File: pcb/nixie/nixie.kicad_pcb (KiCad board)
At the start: 2 copper layers, 144 x 117 mm, 49 parts, among them J1 Conn_01x32, J2 Conn_01x02, J3 Conn_01x32, J4 Conn_01x32, J5 Conn_01x32, P1 TTL_232R_3V3, Q1 Q_NMOS_DGS, U1 LM317EMP, U10 nixie_8422, U11 nixie_8422, U12 nixie_8422, U2 ESP-WROOM-32, U3 TACTILE, U4 TACTILE, U5 nixie_8422, U6 HV5530, U7 HV5530, U8 nixie_8422, U9 nixie_8422

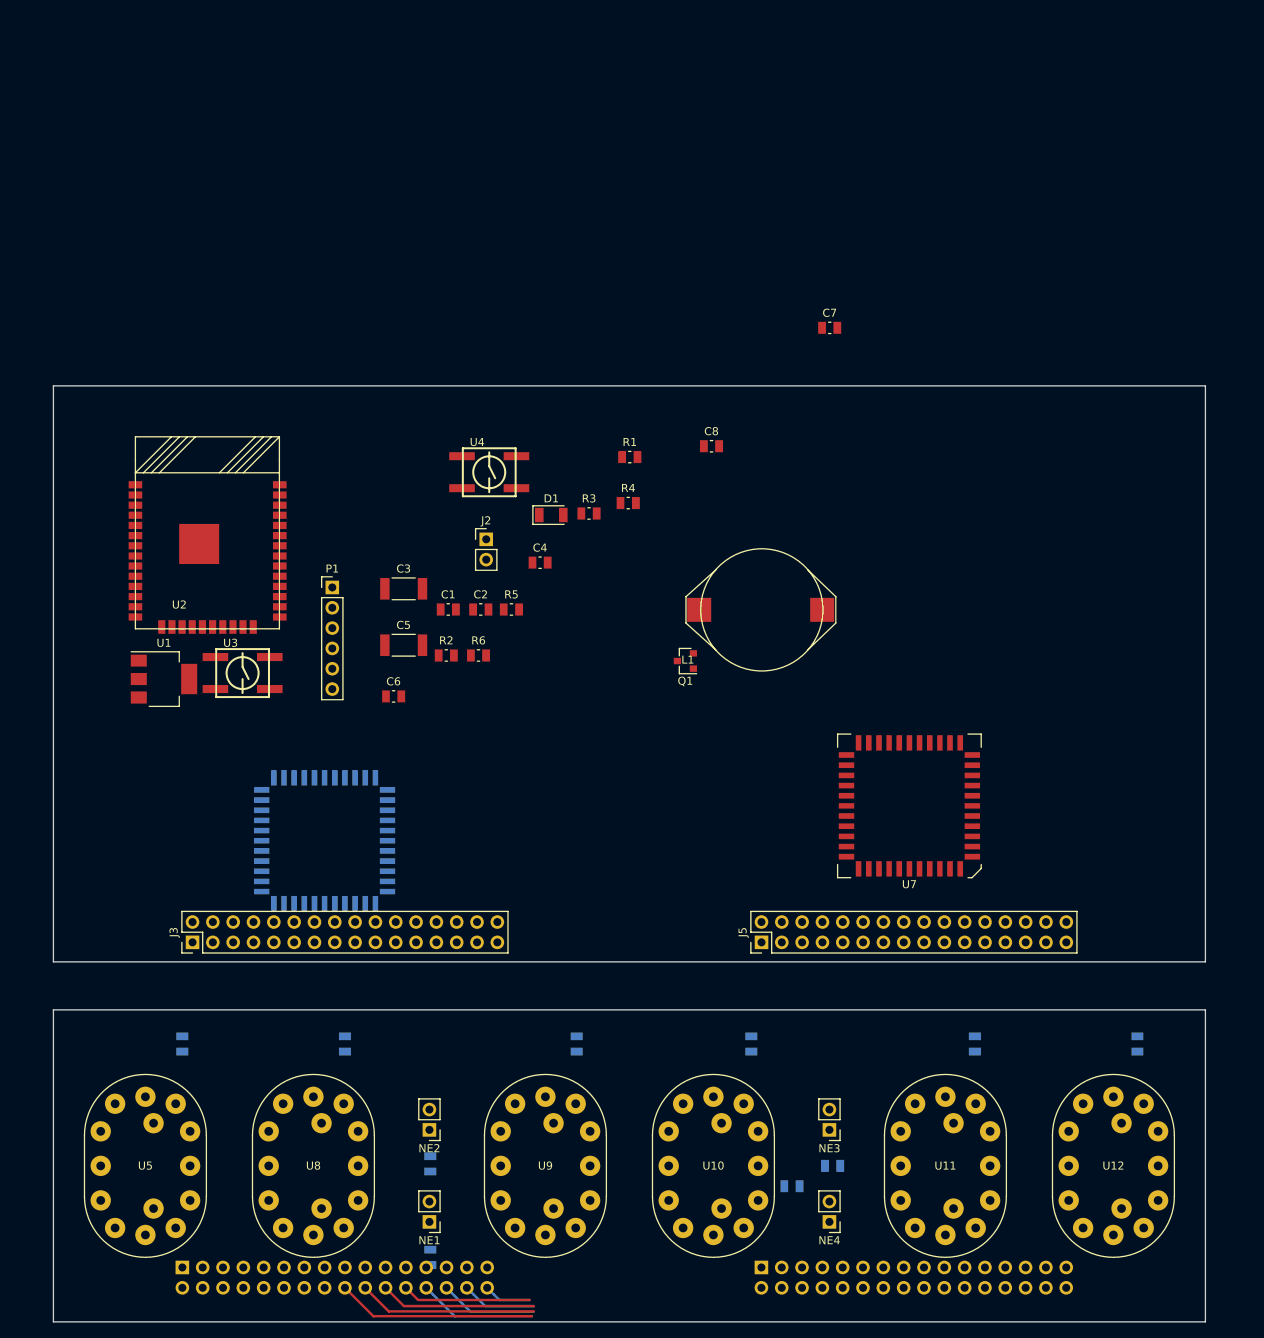
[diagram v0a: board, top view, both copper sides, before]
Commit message: PCB work
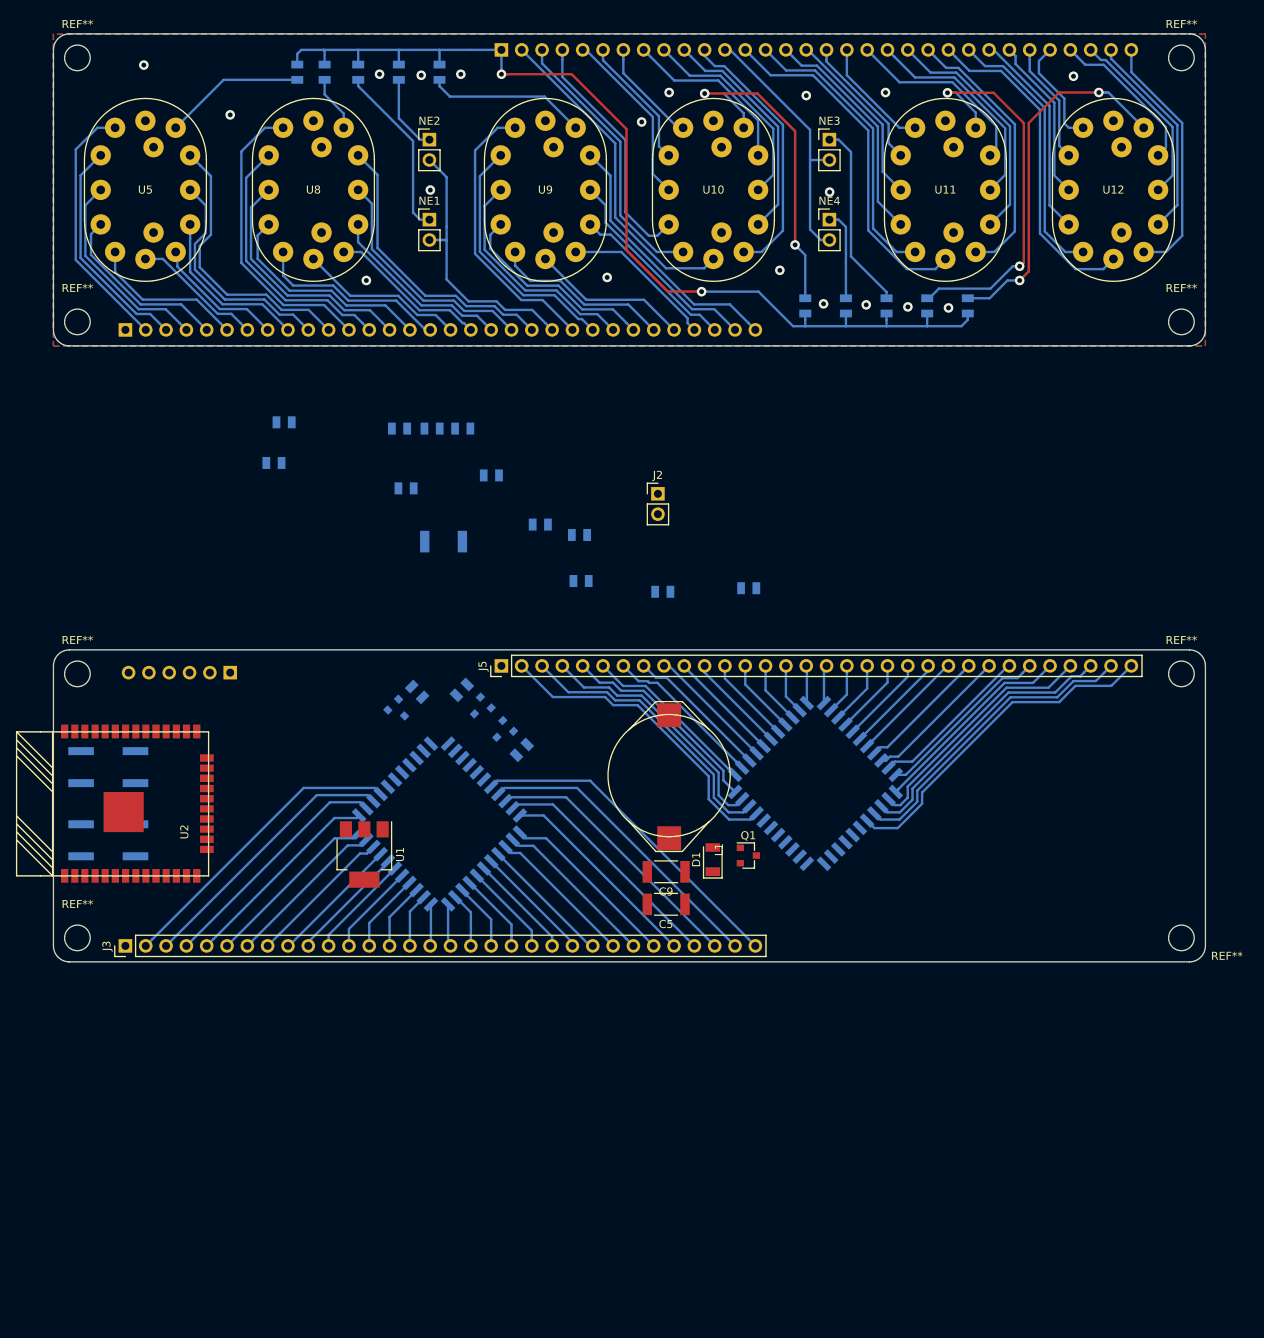
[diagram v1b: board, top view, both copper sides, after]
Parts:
- added C9: 10u, Capacitor_SMD:C_2010_5025Metric, F.Cu at (102.6, 123.7)
- added Q2: 2N7002, Package_TO_SOT_SMD:SOT-23, B.Cu at (79.3, 103.3)
- added Q3: 2N7002, Package_TO_SOT_SMD:SOT-23, B.Cu at (82.1, 106.2)
- added Q4: 2N7002, Package_TO_SOT_SMD:SOT-23, B.Cu at (69.2, 103.5)
- added R17: 1k, Resistor_SMD:R_0805_2012Metric, B.Cu at (77.1, 101.0)
- added R18: 1k, Resistor_SMD:R_0805_2012Metric, B.Cu at (84.5, 108.5)
- added R19: 1k, Resistor_SMD:R_0805_2012Metric, B.Cu at (71.5, 101.3)
- added REF**: MountingHole_3.2mm_M3, MountingHole:MountingHole_3.2mm_M3, F.Cu at (167.0, 99.0)
- added REF**: MountingHole_3.2mm_M3, MountingHole:MountingHole_3.2mm_M3, F.Cu at (29.0, 132.0)
- added REF**: MountingHole_3.2mm_M3, MountingHole:MountingHole_3.2mm_M3, F.Cu at (167.0, 132.0)
- added REF**: MountingHole_3.2mm_M3, MountingHole:MountingHole_3.2mm_M3, F.Cu at (29.0, 99.0)
- added REF**: MountingHole_3.2mm_M3, MountingHole:MountingHole_3.2mm_M3, F.Cu at (29.0, 55.0)
- added REF**: MountingHole_3.2mm_M3, MountingHole:MountingHole_3.2mm_M3, F.Cu at (29.0, 22.0)
- added REF**: MountingHole_3.2mm_M3, MountingHole:MountingHole_3.2mm_M3, F.Cu at (167.0, 55.0)
- added REF**: MountingHole_3.2mm_M3, MountingHole:MountingHole_3.2mm_M3, F.Cu at (167.0, 22.0)
- C1, C2, C3, C4, C6, C7, C8, P1, R1, R2, R3, R4, R5, R6, U3, U4, U7: moved to B.Cu
- J1, J4: footprint Connector_PinHeader_2.54mm:PinHeader_2x16_P2.54mm_Horizontal -> Connector_PinHeader_2.54mm:PinHeader_1x32_P2.54mm_Vertical
- J3, J5: footprint Connector_PinHeader_2.54mm:PinHeader_2x16_P2.54mm_Vertical -> Connector_PinHeader_2.54mm:PinHeader_1x32_P2.54mm_Vertical
- moved J4 155.6 mm to (82.0, 21.0)
- moved R9 148.4 mm to (64.1, 23.8), turned to 270 degrees
- moved R10 136.5 mm to (69.2, 23.8), turned to 270 degrees
- moved NE1 125.3 mm to (73.0, 42.2), turned to 0 degrees
- moved NE4 125.3 mm to (123.0, 42.2), turned to 0 degrees
- moved NE2 123.8 mm to (73.0, 32.2), turned to 0 degrees
- moved NE3 123.8 mm to (123.0, 32.2), turned to 0 degrees
- moved R11 122.7 mm to (74.3, 23.8)
- moved R7 122.3 mm to (56.5, 23.8)
- moved U10 122.0 mm to (108.5, 38.5)
- moved U11 122.0 mm to (137.5, 38.5)
- moved U12 122.0 mm to (158.5, 38.5)
- moved U5 122.0 mm to (37.5, 38.5)
- moved U8 122.0 mm to (58.5, 38.5)
- moved U9 122.0 mm to (87.5, 38.5)
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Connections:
- J1 pad 1: /tubes/n5_0 -> GND
- J1 pad 11: /tubes/n4_0 -> /tubes/n5_0
- J1 pad 21: /tubes/colons_1 -> /tubes/n4_0
- J1 pad 22: /tubes/n3_0 -> /tubes/colons_1
- J1 pad 32: Net-(J1-Pad32) -> /tubes/n3_0
- J3 pad 1: /tubes/n5_0 -> GND
- J3 pad 11: /tubes/n4_0 -> /tubes/n5_0
- J3 pad 21: /tubes/colons_1 -> /tubes/n4_0
- J3 pad 22: /tubes/n3_0 -> /tubes/colons_1
- J3 pad 32: Net-(J3-Pad32) -> /tubes/n3_0
- J4 pad 1: /tubes/n2_0 -> HT
- J4 pad 10: /tubes/n2_9 -> /tubes/n2_8
- J4 pad 11: /tubes/colons_0 -> /tubes/n2_7
- J4 pad 12: /tubes/n1_0 -> /tubes/colons_0
- J4 pad 13: /tubes/n1_1 -> /tubes/n1_6
- J4 pad 14: /tubes/n1_2 -> /tubes/n1_5
- J4 pad 15: /tubes/n1_3 -> /tubes/n1_4
- J4 pad 16: /tubes/n1_4 -> /tubes/n1_3
- J4 pad 17: /tubes/n1_5 -> /tubes/n1_2
- J4 pad 18: /tubes/n1_6 -> /tubes/n1_1
- J4 pad 19: /tubes/n1_7 -> /tubes/n1_0
- J4 pad 2: /tubes/n2_1 -> /tubes/n2_6
- J4 pad 20: /tubes/n1_8 -> /tubes/n1_9
- J4 pad 21: /tubes/n1_9 -> /tubes/n1_8
- J4 pad 22: /tubes/n0_0 -> /tubes/n1_7
- J4 pad 23: /tubes/n0_1 -> /tubes/n0_6
- J4 pad 24: /tubes/n0_2 -> /tubes/n0_5
- J4 pad 25: /tubes/n0_3 -> /tubes/n0_4
- J4 pad 26: /tubes/n0_4 -> /tubes/n0_3
- J4 pad 27: /tubes/n0_5 -> /tubes/n0_2
- J4 pad 28: /tubes/n0_6 -> /tubes/n0_1
- J4 pad 29: /tubes/n0_7 -> /tubes/n0_0
- J4 pad 3: /tubes/n2_2 -> /tubes/n2_5
- J4 pad 30: /tubes/n0_8 -> /tubes/n0_9
- J4 pad 31: /tubes/n0_9 -> /tubes/n0_8
- J4 pad 32: Net-(J4-Pad32) -> /tubes/n0_7
- J4 pad 4: /tubes/n2_3 -> /tubes/n2_4
- J4 pad 5: /tubes/n2_4 -> /tubes/n2_3
- J4 pad 6: /tubes/n2_5 -> /tubes/n2_2
- J4 pad 7: /tubes/n2_6 -> /tubes/n2_1
- J4 pad 8: /tubes/n2_7 -> /tubes/n2_0
- J4 pad 9: /tubes/n2_8 -> /tubes/n2_9
- J5 pad 1: /tubes/n2_0 -> HT
- J5 pad 10: /tubes/n2_9 -> /tubes/n2_8
- J5 pad 11: /tubes/colons_0 -> /tubes/n2_7
- J5 pad 12: /tubes/n1_0 -> /tubes/colons_0
- J5 pad 13: /tubes/n1_1 -> /tubes/n1_6
- J5 pad 14: /tubes/n1_2 -> /tubes/n1_5
- J5 pad 15: /tubes/n1_3 -> /tubes/n1_4
- J5 pad 16: /tubes/n1_4 -> /tubes/n1_3
- J5 pad 17: /tubes/n1_5 -> /tubes/n1_2
- J5 pad 18: /tubes/n1_6 -> /tubes/n1_1
- J5 pad 19: /tubes/n1_7 -> /tubes/n1_0
- J5 pad 2: /tubes/n2_1 -> /tubes/n2_6
- J5 pad 20: /tubes/n1_8 -> /tubes/n1_9
- J5 pad 21: /tubes/n1_9 -> /tubes/n1_8
- J5 pad 22: /tubes/n0_0 -> /tubes/n1_7
- J5 pad 23: /tubes/n0_1 -> /tubes/n0_6
- J5 pad 24: /tubes/n0_2 -> /tubes/n0_5
- J5 pad 25: /tubes/n0_3 -> /tubes/n0_4
- J5 pad 26: /tubes/n0_4 -> /tubes/n0_3
- J5 pad 27: /tubes/n0_5 -> /tubes/n0_2
- J5 pad 28: /tubes/n0_6 -> /tubes/n0_1
- J5 pad 29: /tubes/n0_7 -> /tubes/n0_0
- J5 pad 3: /tubes/n2_2 -> /tubes/n2_5
- J5 pad 30: /tubes/n0_8 -> /tubes/n0_9
- J5 pad 31: /tubes/n0_9 -> /tubes/n0_8
- J5 pad 32: Net-(J5-Pad32) -> /tubes/n0_7
- J5 pad 4: /tubes/n2_3 -> /tubes/n2_4
- J5 pad 5: /tubes/n2_4 -> /tubes/n2_3
- J5 pad 6: /tubes/n2_5 -> /tubes/n2_2
- J5 pad 7: /tubes/n2_6 -> /tubes/n2_1
- J5 pad 8: /tubes/n2_7 -> /tubes/n2_0
- J5 pad 9: /tubes/n2_8 -> /tubes/n2_9
- U2 pad 10: /tubes/clk -> Net-(Q4-Pad1)
- U2 pad 11: /tubes/dat -> Net-(Q3-Pad1)
- U2 pad 12: /tubes/nLatch -> Net-(Q2-Pad1)
- U6 pad 1: /tubes/n4_0 -> /tubes/colons_1
- U6 pad 10: /tubes/n4_9 -> /tubes/n4_2
- U6 pad 11: /tubes/colons_1 -> /tubes/n4_1
- U6 pad 12: /tubes/n3_0 -> /tubes/n5_0
- U6 pad 13: /tubes/n3_1 -> /tubes/n5_9
- U6 pad 14: /tubes/n3_2 -> /tubes/n5_8
- U6 pad 15: /tubes/n3_3 -> /tubes/n5_7
- U6 pad 16: /tubes/n3_4 -> /tubes/n5_6
- U6 pad 17: /tubes/n3_5 -> /tubes/n5_5
- U6 pad 18: /tubes/n3_6 -> /tubes/n5_4
- U6 pad 19: /tubes/n3_7 -> /tubes/n5_3
- U6 pad 2: /tubes/n4_1 -> /tubes/n4_0
- U6 pad 20: /tubes/n3_8 -> /tubes/n5_2
- U6 pad 21: /tubes/n3_9 -> /tubes/n5_1
- U6 pad 3: /tubes/n4_2 -> /tubes/n4_9
- U6 pad 35: /tubes/n5_0 -> /tubes/n3_0
- U6 pad 36: /tubes/n5_1 -> /tubes/n3_9
- U6 pad 37: /tubes/n5_2 -> /tubes/n3_8
- U6 pad 38: /tubes/n5_3 -> /tubes/n3_7
- U6 pad 39: /tubes/n5_4 -> /tubes/n3_6
- U6 pad 4: /tubes/n4_3 -> /tubes/n4_8
- U6 pad 40: /tubes/n5_5 -> /tubes/n3_5
- U6 pad 41: /tubes/n5_6 -> /tubes/n3_4
- U6 pad 42: /tubes/n5_7 -> /tubes/n3_3
- U6 pad 43: /tubes/n5_8 -> /tubes/n3_2
- U6 pad 44: /tubes/n5_9 -> /tubes/n3_1
- U6 pad 5: /tubes/n4_4 -> /tubes/n4_7
- U6 pad 6: /tubes/n4_5 -> /tubes/n4_6
- U6 pad 7: /tubes/n4_6 -> /tubes/n4_5
- U6 pad 8: /tubes/n4_7 -> /tubes/n4_4
- U6 pad 9: /tubes/n4_8 -> /tubes/n4_3
- U7 pad 1: /tubes/colons_0 -> /tubes/n2_7
- U7 pad 10: /tubes/n1_8 -> /tubes/n1_9
- U7 pad 11: /tubes/n1_9 -> /tubes/n1_8
- U7 pad 12: /tubes/n0_0 -> /tubes/n1_7
- U7 pad 13: /tubes/n0_1 -> /tubes/n0_6
- U7 pad 14: /tubes/n0_2 -> /tubes/n0_5
- U7 pad 15: /tubes/n0_3 -> /tubes/n0_4
- U7 pad 16: /tubes/n0_4 -> /tubes/n0_3
- U7 pad 17: /tubes/n0_5 -> /tubes/n0_2
- U7 pad 18: /tubes/n0_6 -> /tubes/n0_1
- U7 pad 19: /tubes/n0_7 -> /tubes/n0_0
- U7 pad 2: /tubes/n1_0 -> /tubes/colons_0
- U7 pad 20: /tubes/n0_8 -> /tubes/n0_9
- U7 pad 21: /tubes/n0_9 -> /tubes/n0_8
- U7 pad 22: Net-(U7-Pad22) -> /tubes/n0_7
- U7 pad 3: /tubes/n1_1 -> /tubes/n1_6
- U7 pad 35: /tubes/n2_0 -> Net-(U7-Pad35)
- U7 pad 36: /tubes/n2_1 -> /tubes/n2_6
- U7 pad 37: /tubes/n2_2 -> /tubes/n2_5
- U7 pad 38: /tubes/n2_3 -> /tubes/n2_4
- U7 pad 39: /tubes/n2_4 -> /tubes/n2_3
- U7 pad 4: /tubes/n1_2 -> /tubes/n1_5
- U7 pad 40: /tubes/n2_5 -> /tubes/n2_2
- U7 pad 41: /tubes/n2_6 -> /tubes/n2_1
- U7 pad 42: /tubes/n2_7 -> /tubes/n2_0
- U7 pad 43: /tubes/n2_8 -> /tubes/n2_9
- U7 pad 44: /tubes/n2_9 -> /tubes/n2_8
- U7 pad 5: /tubes/n1_3 -> /tubes/n1_4
- U7 pad 6: /tubes/n1_4 -> /tubes/n1_3
- U7 pad 7: /tubes/n1_5 -> /tubes/n1_2
- U7 pad 8: /tubes/n1_6 -> /tubes/n1_1
- U7 pad 9: /tubes/n1_7 -> /tubes/n1_0
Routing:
- net HT: track 0.00 -> 125.1 mm, vias 0 -> 2
- net /tubes/n2_6: track 0.00 -> 80.5 mm
- net /tubes/n0_7: track 0.00 -> 74.2 mm
- net /tubes/n5_1: track 0.00 -> 70.1 mm
- net /tubes/n2_5: track 0.00 -> 70.0 mm
- net /tubes/n0_8: track 0.00 -> 64.9 mm
- net /tubes/n3_9: track 0.00 -> 64.7 mm
- net /tubes/n2_4: track 0.00 -> 62.5 mm
- net /tubes/n5_2: track 0.00 -> 62.3 mm
- net /tubes/n0_9: track 0.00 -> 57.7 mm
- net /tubes/n0_6: track 0.00 -> 55.9 mm
- net /tubes/n5_3: track 0.00 -> 55.7 mm
- net /tubes/n3_0: track 19.5 -> 74.9 mm
- net /tubes/n1_6: track 0.00 -> 53.6 mm
- net /tubes/n0_0: track 0.00 -> 50.9 mm
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- added copper zone on B.Cu, net GND
- added copper zone on F.Cu, net GND
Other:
- board size 144 x 117 mm -> 144 x 116 mm
